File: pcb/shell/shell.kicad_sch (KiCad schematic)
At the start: 215 parts, among them J1 Conn_01x11, J2 Conn_01x11

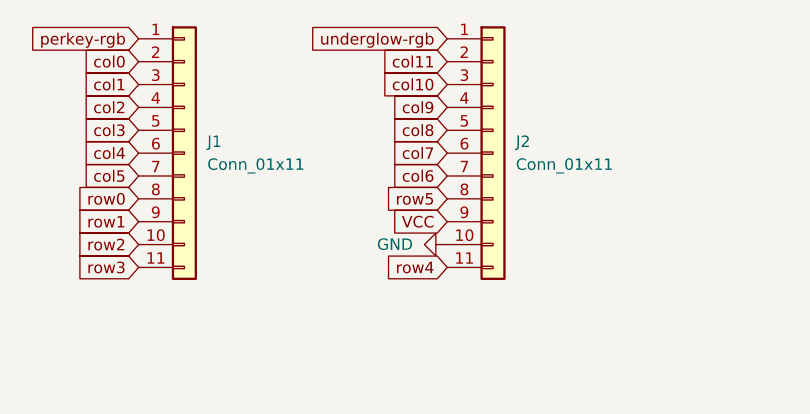
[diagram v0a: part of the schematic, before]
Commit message: finished routing
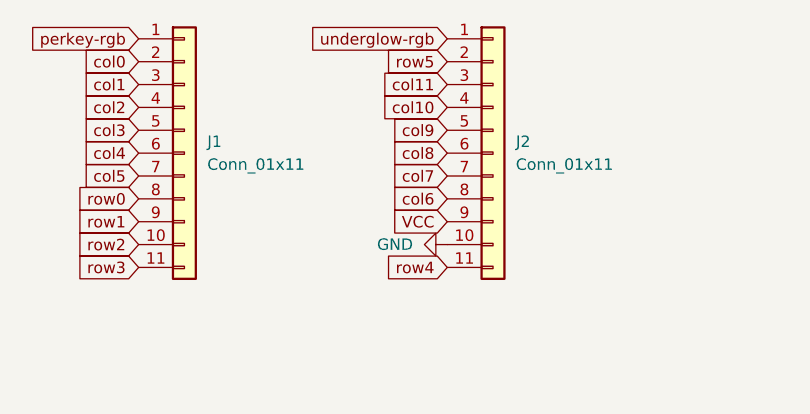
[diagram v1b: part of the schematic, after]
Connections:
- net col10: now also J2.4 (Pin_4); no longer J2.3 (Pin_3)
- net col11: now also J2.3 (Pin_3); no longer J2.2 (Pin_2)
- net col6: now also J2.8 (Pin_8); no longer J2.7 (Pin_7)
- net col7: now also J2.7 (Pin_7); no longer J2.6 (Pin_6)
- net col8: now also J2.6 (Pin_6); no longer J2.5 (Pin_5)
- net col9: now also J2.5 (Pin_5); no longer J2.4 (Pin_4)
- net row5: now also J2.2 (Pin_2); no longer J2.8 (Pin_8)
